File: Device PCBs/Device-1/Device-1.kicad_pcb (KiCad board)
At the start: 2 copper layers, 55 x 55 mm, 36 parts, among them J1 Conn_01x04_Female, J2 Conn_01x04_Female, U1 EBYTE_E32-433T20D, U2 MAX487E

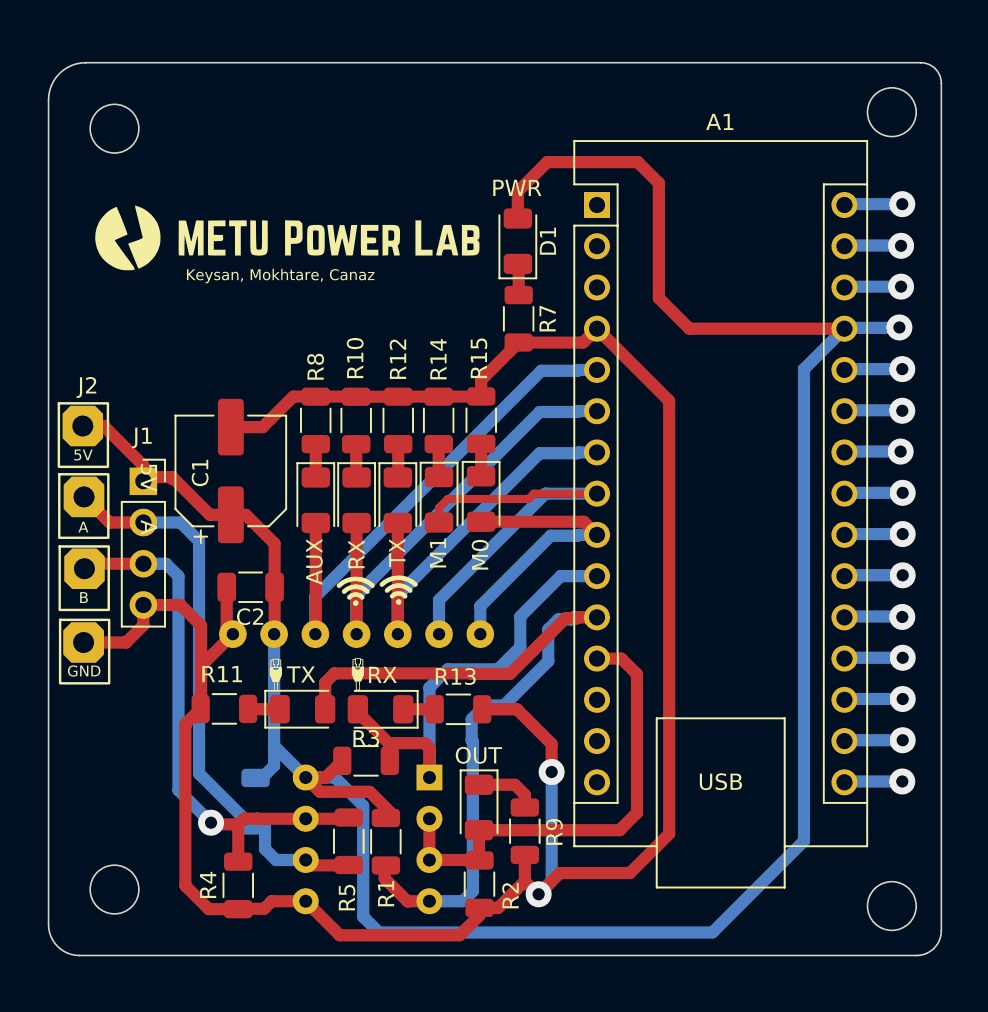
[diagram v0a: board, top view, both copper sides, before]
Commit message: Device 1 PCB is finished
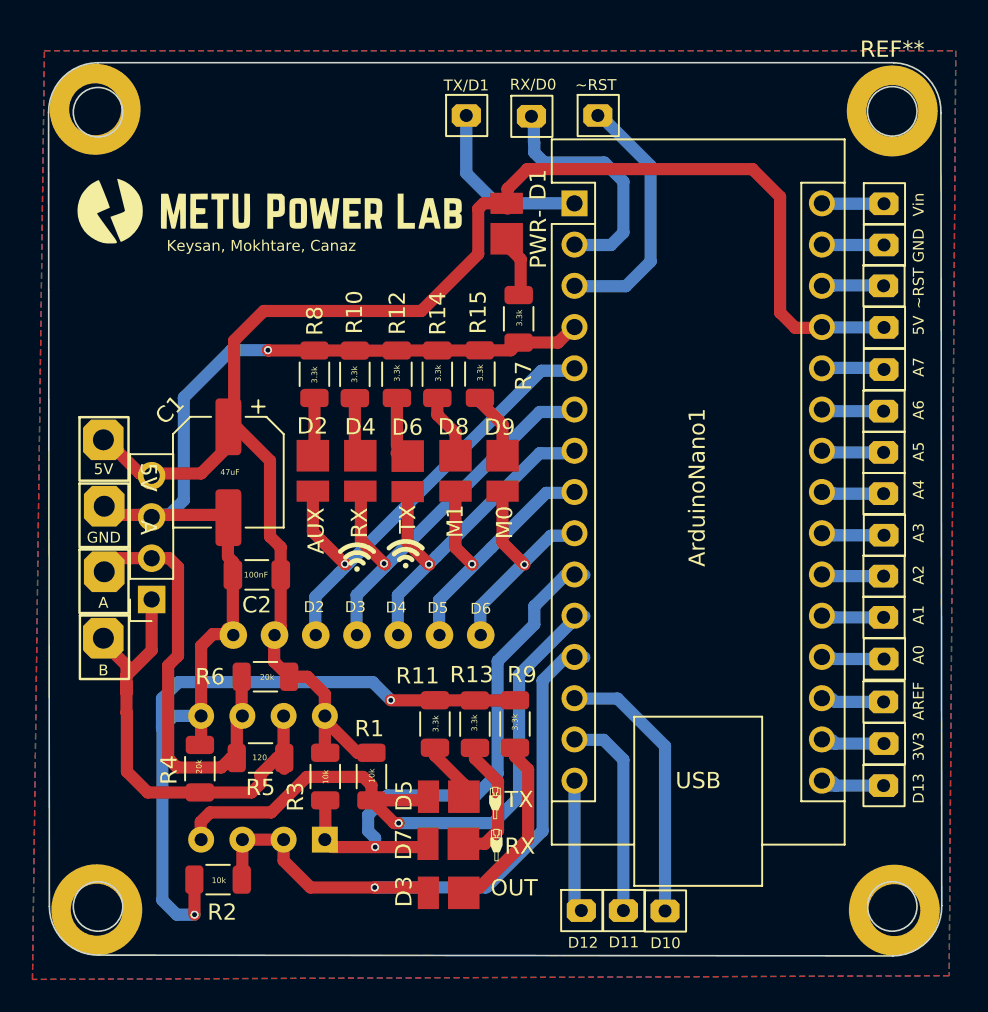
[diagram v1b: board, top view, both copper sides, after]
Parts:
- removed the G*** at (32.0, 50.6)
- removed the G*** at (26.9, 50.6)
- added ?: , , F.Cu at (15.9, 65.1)
- added ?: , , F.Cu at (15.8, 15.8)
- added ?: , , F.Cu at (65.0, 65.2)
- added G***: LOGO, LOGO, F.Cu at (40.5, 58.5)
- added G***: LOGO, LOGO, F.Cu at (40.5, 61.1)
- added REF**: MountingHole_3.2mm_M3_DIN965_Pad, MountingHole:MountingHole_3.2mm_M3_DIN965_Pad, F.Cu at (64.9, 15.9)
- added U10: signle_via, Device_1_project_footprints:single_via, F.Cu at (64.4, 52.3)
- added U11: signle_via, Device_1_project_footprints:single_via, F.Cu at (64.4, 49.7)
- added U12: signle_via, Device_1_project_footprints:single_via, F.Cu at (64.4, 47.1)
- added U13: signle_via, Device_1_project_footprints:single_via, F.Cu at (64.4, 44.6)
- added U14: signle_via, Device_1_project_footprints:single_via, F.Cu at (64.4, 42.0)
- added U15: signle_via, Device_1_project_footprints:single_via, F.Cu at (64.4, 39.5)
- added U16: signle_via, Device_1_project_footprints:single_via, F.Cu at (64.4, 36.9)
- added U17: signle_via, Device_1_project_footprints:single_via, F.Cu at (64.4, 34.4)
- added U18: signle_via, Device_1_project_footprints:single_via, F.Cu at (64.4, 31.8)
- added U19: signle_via, Device_1_project_footprints:single_via, F.Cu at (64.4, 21.6)
- added U20: signle_via, Device_1_project_footprints:single_via, F.Cu at (64.4, 29.2)
- added U21: signle_via, Device_1_project_footprints:single_via, F.Cu at (64.4, 54.9)
- added U22: signle_via, Device_1_project_footprints:single_via, F.Cu at (38.7, 16.2)
- added U23: signle_via, Device_1_project_footprints:single_via, F.Cu at (42.7, 16.2)
- added U3: signle_via, Device_1_project_footprints:single_via, F.Cu at (50.9, 65.2)
- added U4: signle_via, Device_1_project_footprints:single_via, F.Cu at (48.3, 65.2)
- added U5: signle_via, Device_1_project_footprints:single_via, F.Cu at (45.7, 65.2)
- added U6: signle_via, Device_1_project_footprints:single_via, F.Cu at (64.4, 57.5)
- added U7: signle_via, Device_1_project_footprints:single_via, F.Cu at (64.4, 24.2)
- added U8: signle_via, Device_1_project_footprints:single_via, F.Cu at (64.4, 26.7)
- added U9: signle_via, Device_1_project_footprints:single_via, F.Cu at (46.8, 16.2)
- C1: footprint Capacitor_SMD:CP_Elec_6.3x5.7 -> Capacitor_SMD:CP_Elec_6.3x5.2
- D1, D2, D3, D8, D9: footprint LED_SMD:LED_1206_3216Metric -> Device_1_project_footprints:lm281B-3000K
- D4, D5, D6, D7: footprint LED_SMD:LED_1206_3216Metric -> Device_1_project_footprints:lm281B-6500K
- R6: moved to F.Cu
- moved R2 16.1 mm to (23.4, 63.3), turned to 0 degrees
- moved R11 13.0 mm to (36.8, 53.7), turned to 90 degrees
- moved D5 10.9 mm to (37.6, 58.9)
- moved D7 9.98 mm to (37.6, 61.8), turned to 0 degrees
- moved R6 7.72 mm to (26.3, 50.8), turned to 0 degrees
- moved R4 7.57 mm to (22.3, 56.4), turned to -90 degrees
- moved U2 7.49 mm to (30.0, 60.8), turned to 90 degrees
- moved R5 7.47 mm to (26.0, 55.8), turned to 180 degrees
- moved J1 7.30 mm to (19.3, 46.0), turned to 180 degrees
- moved R9 6.63 mm to (41.7, 53.7), turned to 90 degrees
- moved D3 5.60 mm to (37.3, 64.0), turned to 0 degrees
- moved R1 4.11 mm to (32.8, 56.9)
- moved R12 2.84 mm to (34.4, 32.1)
- moved R14 2.84 mm to (36.9, 32.1)
- moved R15 2.84 mm to (39.5, 32.1)
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- renumbered A1 to ArduinoNano1
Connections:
- ArduinoNano1 pad 1: unconnected-(A1-Pad1) -> Net-(ArduinoNano1-Pad1)
- ArduinoNano1 pad 13: unconnected-(A1-Pad13) -> Net-(ArduinoNano1-Pad13)
- ArduinoNano1 pad 14: unconnected-(A1-Pad14) -> Net-(ArduinoNano1-Pad14)
- ArduinoNano1 pad 15: unconnected-(A1-Pad15) -> Net-(ArduinoNano1-Pad15)
- ArduinoNano1 pad 16: unconnected-(A1-Pad16) -> Net-(ArduinoNano1-Pad16)
- ArduinoNano1 pad 17: unconnected-(A1-Pad17) -> Net-(ArduinoNano1-Pad17)
- ArduinoNano1 pad 18: unconnected-(A1-Pad18) -> Net-(ArduinoNano1-Pad18)
- ArduinoNano1 pad 19: unconnected-(A1-Pad19) -> Net-(ArduinoNano1-Pad19)
- ArduinoNano1 pad 2: unconnected-(A1-Pad2) -> Net-(ArduinoNano1-Pad2)
- ArduinoNano1 pad 20: unconnected-(A1-Pad20) -> Net-(ArduinoNano1-Pad20)
- ArduinoNano1 pad 21: unconnected-(A1-Pad21) -> Net-(ArduinoNano1-Pad21)
- ArduinoNano1 pad 22: unconnected-(A1-Pad22) -> Net-(ArduinoNano1-Pad22)
- ArduinoNano1 pad 23: unconnected-(A1-Pad23) -> Net-(ArduinoNano1-Pad23)
- ArduinoNano1 pad 24: unconnected-(A1-Pad24) -> Net-(ArduinoNano1-Pad24)
- ArduinoNano1 pad 25: unconnected-(A1-Pad25) -> Net-(ArduinoNano1-Pad25)
- ArduinoNano1 pad 26: unconnected-(A1-Pad26) -> Net-(ArduinoNano1-Pad26)
- ArduinoNano1 pad 28: unconnected-(A1-Pad28) -> Net-(ArduinoNano1-Pad28)
- ArduinoNano1 pad 29: unconnected-(A1-Pad29) -> Net-(ArduinoNano1-Pad29)
- ArduinoNano1 pad 3: unconnected-(A1-Pad3) -> Net-(ArduinoNano1-Pad3)
- ArduinoNano1 pad 30: unconnected-(A1-Pad30) -> Net-(ArduinoNano1-Pad30)
- J1 pad 1: 5V -> B
- J1 pad 3: B -> GND
- J1 pad 4: GND -> 5V
- J2 pad 1: GND -> B
- J2 pad 2: B -> A
- J2 pad 3: A -> GND
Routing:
- net 5V: track 151.3 -> 97.7 mm, vias 1 -> 0
- net GND: track 141.9 -> 102.9 mm, vias 2 -> 3
- net Net-(ArduinoNano1-Pad13): track 0.00 -> 16.3 mm
- net Net-(ArduinoNano1-Pad3): track 0.00 -> 14.9 mm
- net Net-(ArduinoNano1-Pad2): track 0.00 -> 14.4 mm
- net Net-(ArduinoNano1-Pad14): track 0.00 -> 12.2 mm
- net RS485_OUTPUT_ENABLE_PIN: track 29.1 -> 40.2 mm, vias 0 -> 1
- net Net-(ArduinoNano1-Pad1): track 0.00 -> 11.0 mm
- net Net-(ArduinoNano1-Pad15): track 0.00 -> 8.44 mm
- net RS485_SS_TX_PIN: track 49.3 -> 40.9 mm, vias 0 -> 1
- net M1: track 25.6 -> 18.1 mm, vias 0 -> 1
- net A: track 34.6 -> 27.3 mm
- net RS485_SS_RX_PIN: track 28.3 -> 35.4 mm, vias 0 -> 1
- net Net-(D3-Pad1): track 4.07 -> 11.1 mm
- net Net-(D7-Pad1): track 1.94 -> 8.18 mm
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- added copper zone on B.Cu, net GND
- added copper zone on F.Cu, net GND
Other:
- outline, holes or cut-outs redrawn
- board text added: "100nF"
- board text added: "10k"
- board text added: "120"
- board text added: "20k"
- board text added: "3.3k"
- board text added: "3V3"
- board text added: "47uF"
- board text added: "A0"
- board text added: "A1"
- board text added: "A2"
- board text added: "A3"
- board text added: "A4"
- board text added: "A5"
- board text added: "A6"
- board text added: "A7"
- board text added: "AREF"
- board text added: "D10"
- board text added: "D11"
- board text added: "D12"
- board text added: "D13"
- board text added: "D2"
- board text added: "D3"
- board text added: "D4"
- board text added: "D5"
- board text added: "D6"
- board text added: "Designed by Erdem Canaz 27.02.2023 github.com/erdemcanaz"
- board text added: "EBYTE-E32"
- board text added: "GND"
- board text added: "MAX487"
- board text added: "PWR-"
- board text added: "RX/D0"
- board text added: "TX/D1"
- board text added: "Vin"
- board text added: "~RST"
- board text removed: "PWR"
